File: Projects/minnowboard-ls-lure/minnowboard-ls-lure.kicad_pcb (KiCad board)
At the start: 2 copper layers, 99.1 x 73.7 mm, 5 parts, among them P1 CONN_02X13

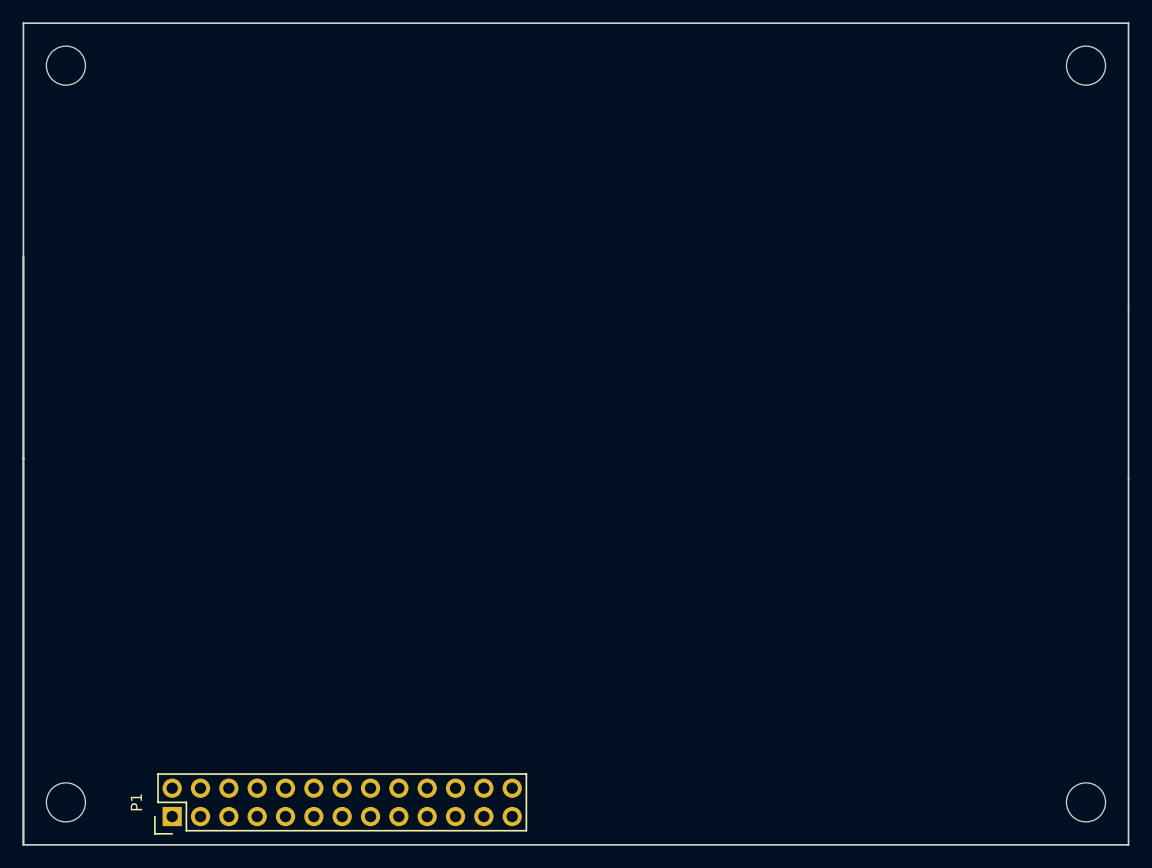
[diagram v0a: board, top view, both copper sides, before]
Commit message: Update existing templates to version 6
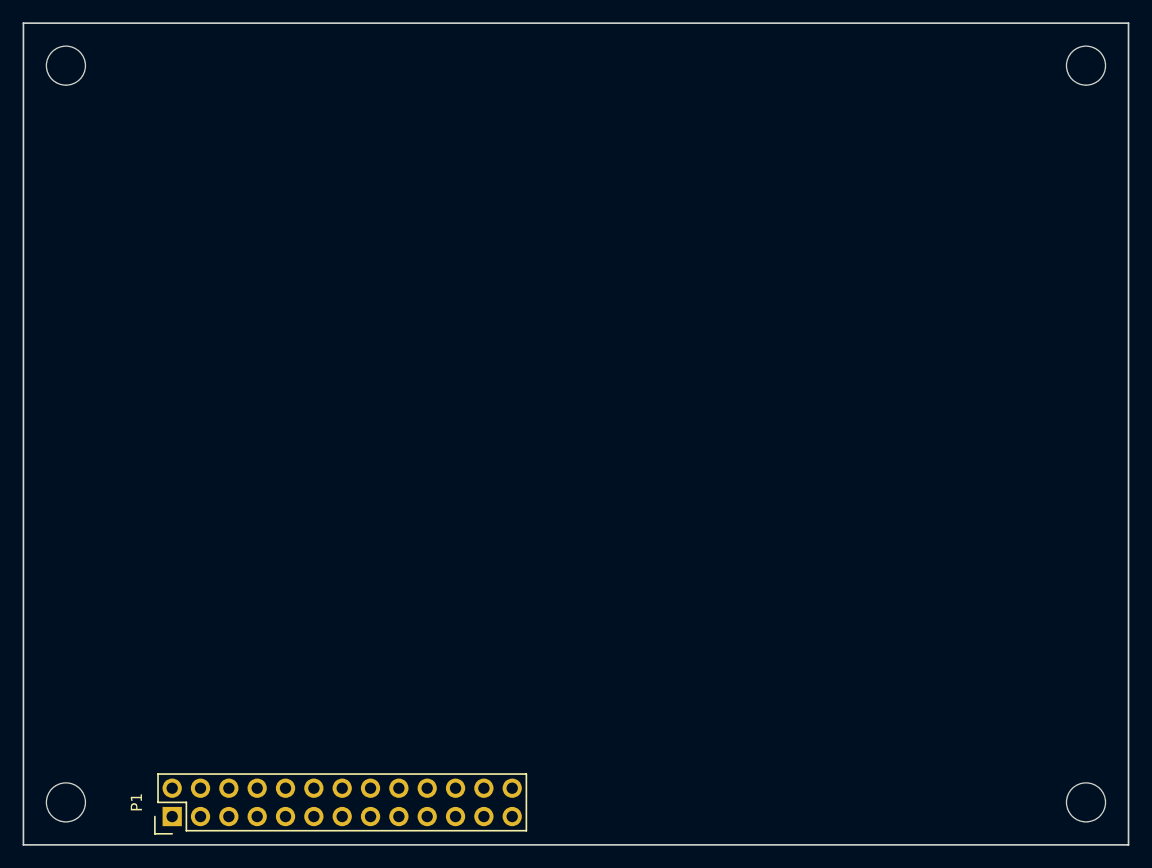
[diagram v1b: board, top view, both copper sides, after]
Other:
- outline, holes or cut-outs redrawn
- net class Default removed
- board text removed: "NOTE: NO BOTTOM SIDE OR THROUGH-HOLE COMPONENTS IN THE AREAS DESIGNATED IN THE DWGS.USER LAYER TO AVOID COLLISION WITH MINNOWBOARD ETHERNET AND USB CONNECTORS."
